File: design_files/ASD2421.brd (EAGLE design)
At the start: 22.5 x 22.5 mm, 12 parts, among them J2 DF12-32-DS

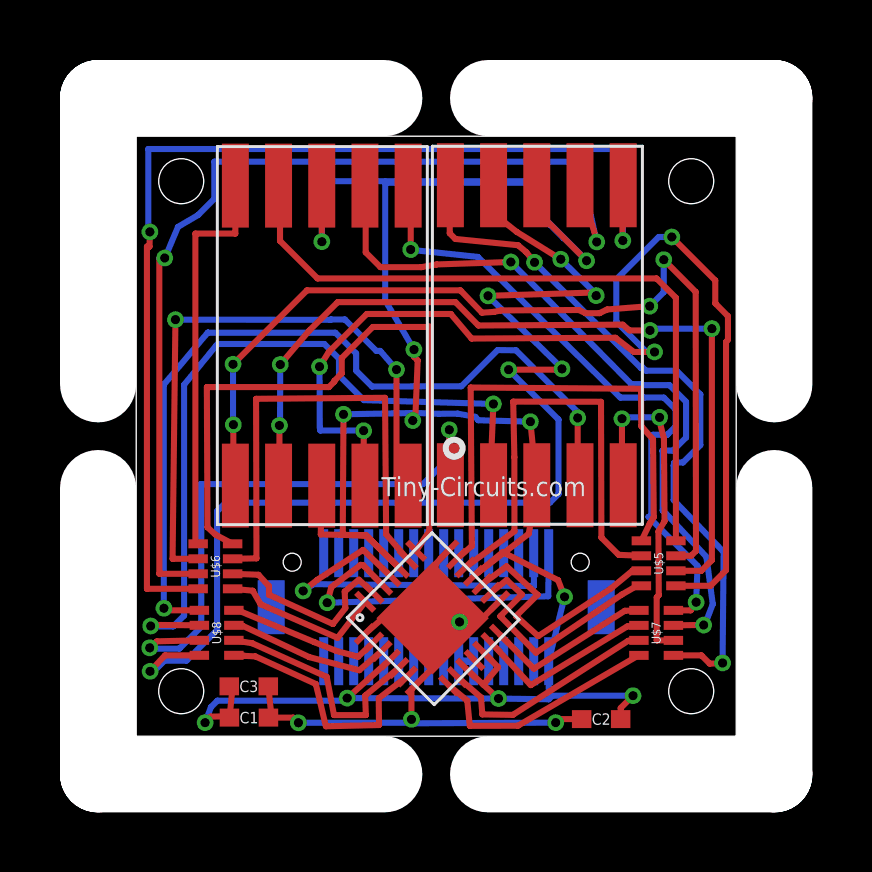
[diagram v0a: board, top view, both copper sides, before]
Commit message: Update Rev and Format
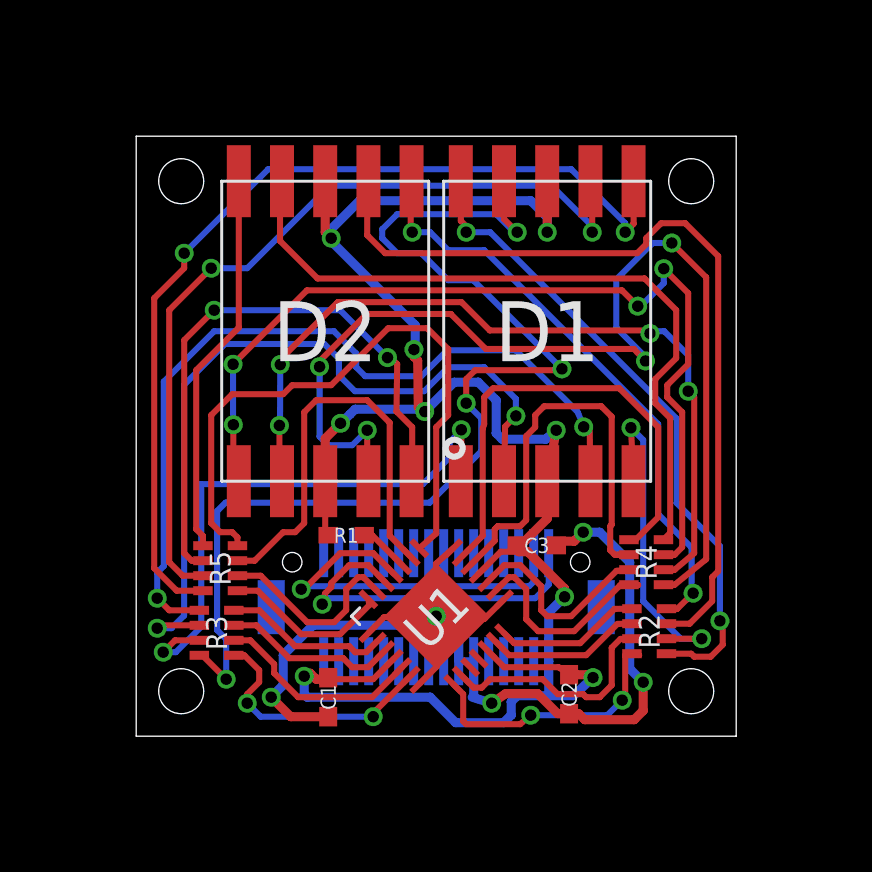
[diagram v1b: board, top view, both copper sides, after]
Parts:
- removed U$2, U$3: AS-ITM-00133, tinycircuits:ACSA02-41SURKWA-F01
- removed U$4: AS-ITM-00134, tinycircuits:SX1506
- removed U$5, U$6, U$7: AS-ITM-00135, tinycircuits:0402RPACK
- added D1, D2: ACSA02-41SURKWA-F01, tinycircuits:ACSA02-41SURKWA-F01
- added R1: 10.0K, tinycircuits:0402
- added R2, R4, R5: 330, tinycircuits:0402RPACK
- added U1: SX1506, tinycircuits:SX1506
- R3: value AS-ITM-00135 -> 330
- moved C3 10.7 mm to (23.4, 16.4)
- moved C1 2.73 mm to (16.4, 11.3), turned to 270 degrees
- moved C2 1.35 mm to (24.4, 11.4), turned to 270 degrees
- renumbered U$8 to R3
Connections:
- new net RST: R1.1, U1.24
- net AD4/SDA: now also U1.25; no longer U$4.25
- net AD5/SCL: now also U1.26; no longer U$4.26
- net GND: now also U1.1, U1.15, U1.21, U1.29, U1.7; no longer U$4.1, U$4.15, U$4.21, U$4.29, U$4.7
- net GPIO0: now also D1.7, R5.6; no longer U$2.7, U$6.6
- net GPIO1: now also D1.6, R5.8; no longer U$2.6, U$6.8
- net GPIO10: now also D2.4, R4.2; no longer U$3.4, U$5.2
- net GPIO11: now also D2.2, R4.4; no longer U$3.2, U$5.4
- net GPIO12: now also D2.1, R4.6; no longer U$3.1, U$5.6
- net GPIO13: now also D2.9, R4.8; no longer U$3.9, U$5.8
- net GPIO14: now also D2.10, R5.2; no longer U$3.10, U$6.2
- net GPIO15: now also D2.5, R5.4; no longer U$3.5, U$6.4
- net GPIO2: now also D1.4; no longer U$2.4
- net GPIO3: now also D1.2; no longer U$2.2
- net GPIO4: now also D1.1; no longer U$2.1
- net GPIO5: now also D1.9; no longer U$2.9
- net GPIO6: now also D1.10, R2.7; no longer U$2.10, U$7.7
- net GPIO7: now also D1.5, R2.5; no longer U$2.5, U$7.5
- net GPIO8: now also D2.7, R2.3; no longer U$3.7, U$7.3
- net GPIO9: now also D2.6, R2.1; no longer U$3.6, U$7.1
- net N$1: now also R2.2, U1.14; no longer U$4.14, U$7.2
- net N$10: now also U1.2; no longer U$4.2
- net N$19: now also R4.1, U1.16; no longer U$4.16, U$5.1
- net N$2: now also R2.4, U1.13; no longer U$4.13, U$7.4
- net N$20: now also R4.3, U1.17; no longer U$4.17, U$5.3
- net N$21: now also R4.5, U1.19; no longer U$4.19, U$5.5
- net N$22: now also R4.7, U1.20; no longer U$4.20, U$5.7
- net N$23: now also R5.1, U1.22; no longer U$4.22, U$6.1
- net N$24: now also R5.3, U1.23; no longer U$4.23, U$6.3
- net N$25: now also R5.5, U1.27; no longer U$4.27, U$6.5
- net N$26: now also R5.7, U1.28; no longer U$4.28, U$6.7
- net N$3: now also R2.6, U1.9; no longer U$4.9, U$7.6
- net N$4: now also R2.8, U1.8; no longer U$4.8, U$7.8
- net N$6: now also U1.6; no longer U$4.6
- net N$7: now also U1.5; no longer U$4.5
- net N$9: now also U1.3; no longer U$4.3
- net VCC: now also D1.3, D1.8, D2.3, D2.8, R1.2, U1.12, U1.18, U1.4; no longer U$2.3, U$2.8, U$3.3, U$3.8, U$4.10, U$4.12, U$4.18, U$4.24, U$4.4
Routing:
- net VCC: track 88.0 -> 64.4 mm, vias 11 -> 9
- net GND: track 24.7 -> 37.9 mm, vias 4 -> 5
- net GPIO1: track 37.2 -> 31.6 mm
- net GPIO0: track 32.8 -> 28.0 mm
- net GPIO8: track 24.7 -> 28.2 mm, vias 2 -> 0
- net GPIO6: track 24.1 -> 21.6 mm
- net GPIO5: track 39.6 -> 37.5 mm, vias 6 -> 4
- net GPIO9: track 21.8 -> 19.8 mm
- net N$20: track 8.55 -> 6.76 mm
- net RST: track 0.00 -> 1.68 mm
- net N$24: track 16.1 -> 14.5 mm
- net GPIO11: track 28.8 -> 27.4 mm
- net N$4: track 7.93 -> 9.29 mm, vias 0 -> 2
- net N$19: track 8.30 -> 7.21 mm
- net N$2: track 6.07 -> 5.16 mm
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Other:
- board size 22.5 x 22.5 mm -> 20 x 20 mm
- board text added: "2"
- board text added: "ASD2421 - Rev2"
- board text added: "TinyCircuits.com"
- board text removed: "1"
- board text removed: "ASD2421 - Rev1"
- board text removed: "Tiny-Circuits.com"
